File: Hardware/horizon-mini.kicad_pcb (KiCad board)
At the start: 2 copper layers, 34 x 41.8 mm, 91 parts, among them J1 Screw_Terminal_01x02, J16 arming terminal, J2 Conn_01x02_Pin, J3 Micro_SD_Card_Det1, J7 USB_C_Receptacle_USB2.0_16P, J8 Conn_02x03_Counter_Clockwise, Q1 BSS138, Q10 DMG2301L, Q2 IRLML6402, U1 TPS82130, U16 AP2112K-3.3, U2 TPS61092, U3 LTC4412xS6, U5 ATSAMD21G18A-A, U6 NAND, U7 LPS22HB, U9 LSM6DS3

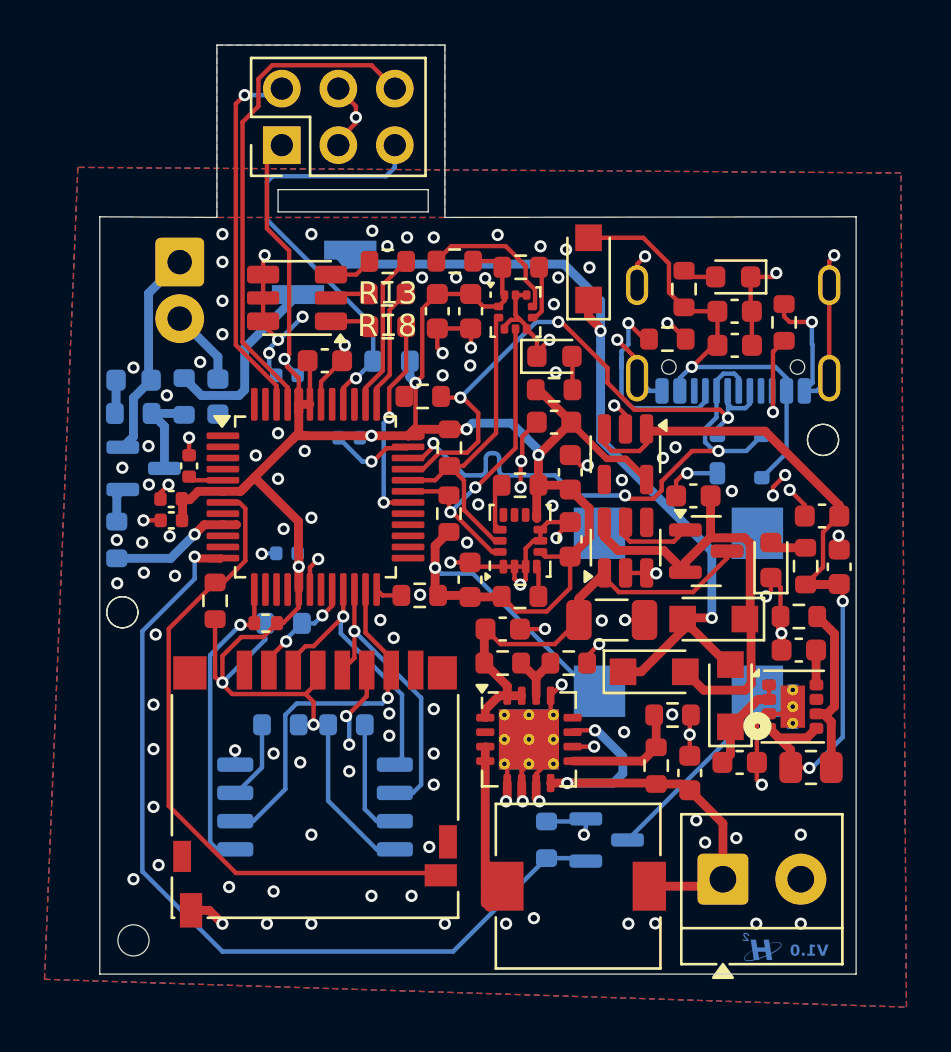
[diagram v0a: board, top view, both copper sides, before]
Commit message: @mpkendall please review before ordering.
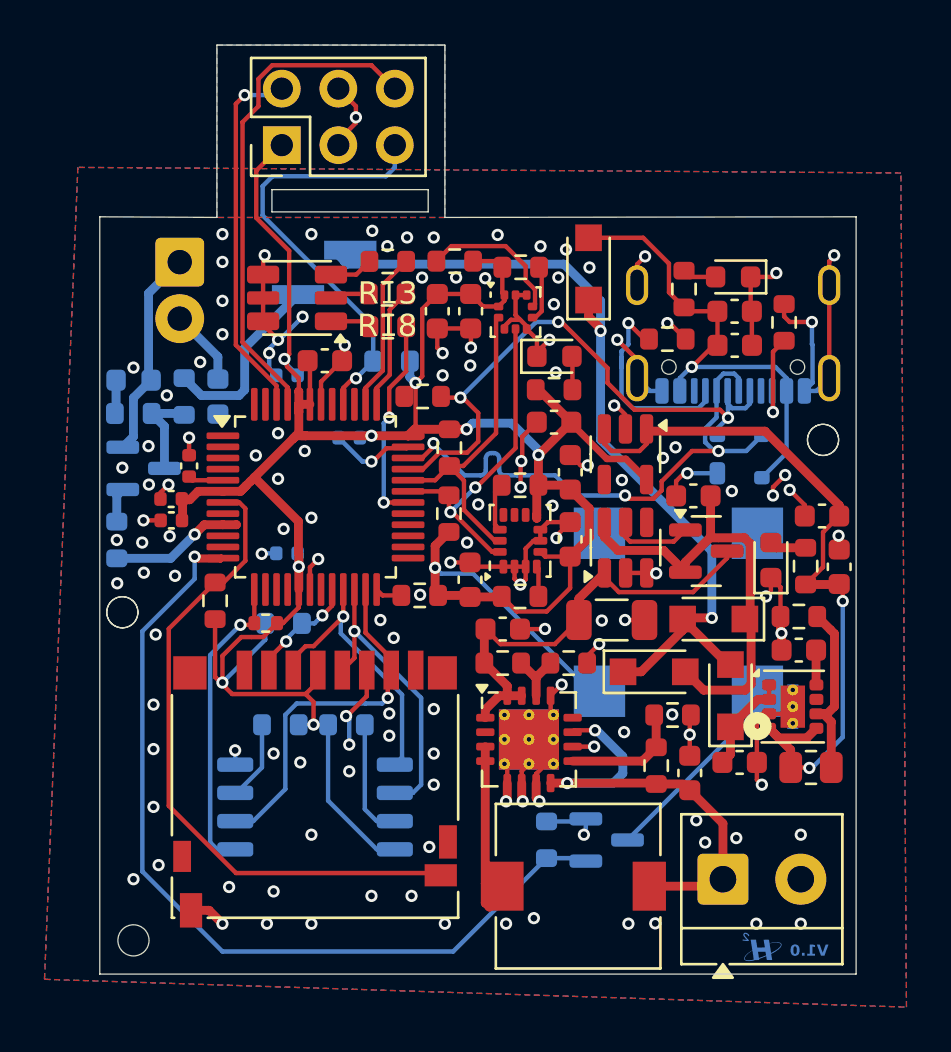
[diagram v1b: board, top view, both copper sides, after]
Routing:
- net GND: track 107.8 -> 110.8 mm
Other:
- outline, holes or cut-outs redrawn
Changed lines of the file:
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@@
 	)
 	(gr_rect
-		(start 144 101.25)
+		(start 143.724967 101.25)
 		(end 150.75 102.25)
 		(stroke
@@
 	)
 	(segment
+		(start 143.021263 100.398737)
+		(end 144.17 99.25)
+		(width 0.2)
+		(layer "F.Cu")
+		(net 1)
+	)
+	(segment
 		(start 145.4325 109.044259)
 		(end 145.328526 108.940285)
@@
 	)
 	(segment
-		(start 144.501 104)
-		(end 143.5 102.999)
-		(width 0.2)
-		(layer "F.Cu")
-		(net 1)
-	)
-	(segment
 		(start 145.7875 123.377)
 		(end 145.2385 123.926)
@@
 	)
 	(segment
-		(start 144.287495 108.863018)
-		(end 144.501 108.649513)
-		(width 0.2)
-		(layer "F.Cu")
-		(net 1)
-	)
-	(segment
 		(start 139.708542 115.190285)
 		(end 139.67448 115.156223)
@@
 	)
 	(segment
-		(start 143.5 99.92)
-		(end 144.17 99.25)
-		(width 0.2)
-		(layer "F.Cu")
-		(net 1)
-	)
-	(segment
 		(start 153.914161 106.502854)
 		(end 153.220573 106.502854)
@@
 	)
 	(segment
+		(start 144.501 108.649513)
+		(end 144.501 104)
+		(width 0.2)
+		(layer "F.Cu")
+		(net 1)
+	)
+	(segment
+		(start 144.287495 108.863018)
+		(end 144.501 108.649513)
+		(width 0.2)
+		(layer "F.Cu")
+		(net 1)
+	)
+	(segment
 		(start 144.9325 117.597446)
 		(end 144.917527 117.582473)
@@
 	)
 	(segment
+		(start 144.501 104)
+		(end 143.021263 102.520263)
+		(width 0.2)
+		(layer "F.Cu")
+		(net 1)
+	)
+	(segment
 		(start 144.224737 120.739203)
 		(end 144.9325 120.03144)
@@
 	)
 	(segment
+		(start 143.021263 102.520263)
+		(end 143.021263 100.398737)
+		(width 0.2)
+		(layer "F.Cu")
+		(net 1)
+	)
+	(segment
 		(start 157.1307 119.159349)
 		(end 157.1307 117.747383)
@@
 	)
 	(segment
-		(start 143.5 102.999)
-		(end 143.5 99.92)
-		(width 0.2)
-		(layer "F.Cu")
-		(net 1)
-	)
-	(segment
 		(start 149.845 112.314848)
 		(end 150.135518 112.02433)
@@
 	)
 	(segment
-		(start 144.501 108.649513)
-		(end 144.501 104)
-		(width 0.2)
-		(layer "F.Cu")
-		(net 1)
-	)
-	(segment
 		(start 144.9325 111.25)
 		(end 144.9325 110.902348)
@@
 	)
 	(segment
+		(start 167.140253 123.742122)
+		(end 167.140253 125.242122)
+		(width 0.2)
+		(layer "F.Cu")
+		(net 2)
+	)
+	(segment
 		(start 167 107.2)
 		(end 166.75 106.95)
@@
 	)
 	(segment
+		(start 167.140253 124.492122)
+		(end 167.140253 125.242122)
+		(width 0.2)
+		(layer "B.Cu")
+		(net 2)
+	)
+	(segment
 		(start 146.72 112.4)
 		(end 147.792635 113.472635)
@@
 	)
 	(segment
+		(start 167.140253 123.742122)
+		(end 167.140253 124.492122)
+		(width 0.2)
+		(layer "B.Cu")
+		(net 2)
+	)
+	(segment
 		(start 168.027249 108.227249)
 		(end 168.027249 109.933323)
@@
 	)
 	(segment
-		(start 143.501292 100.898766)
-		(end 143.751058 100.649)
+		(start 148.275746 107.375688)
+		(end 143.307957 102.407899)
 		(width 0.2)
 		(layer "B.Cu")
@@
 	)
 	(segment
-		(start 149.25 100.25)
-		(end 149.25 99.25)
+		(start 148.275746 108.960863)
+		(end 148.275746 107.375688)
 		(width 0.2)
 		(layer "B.Cu")
@@
 	)
 	(segment
-		(start 148.851 100.649)
-		(end 149.25 100.25)
+		(start 143.307957 102.407899)
+		(end 143.307957 101.092101)
 		(width 0.2)
 		(layer "B.Cu")
@@
 	)
 	(segment
-		(start 148.275746 107.375688)
-		(end 143.501292 102.601234)
+		(start 148.851 100.649)
+		(end 149.25 100.25)
 		(width 0.2)
 		(layer "B.Cu")
@@
 	)
 	(segment
-		(start 148.275746 108.960863)
-		(end 148.275746 107.375688)
+		(start 143.307957 101.092101)
+		(end 143.751058 100.649)
 		(width 0.2)
 		(layer "B.Cu")
@@
 	)
 	(segment
-		(start 147.504561 109.732048)
-		(end 148.275746 108.960863)
+		(start 149.25 100.25)
+		(end 149.25 99.25)
 		(width 0.2)
 		(layer "B.Cu")
@@
 	)
 	(segment
-		(start 143.501292 102.601234)
-		(end 143.501292 100.898766)
+		(start 147.504561 109.732048)
+		(end 148.275746 108.960863)
 		(width 0.2)
 		(layer "B.Cu")
